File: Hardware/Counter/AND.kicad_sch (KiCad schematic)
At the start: 6 parts, among them Q105 FDN360P, Q106 FDN335N, Q107 FDN335N, Q108 FDN335N, U60 FDN360P, U61 FDN360P

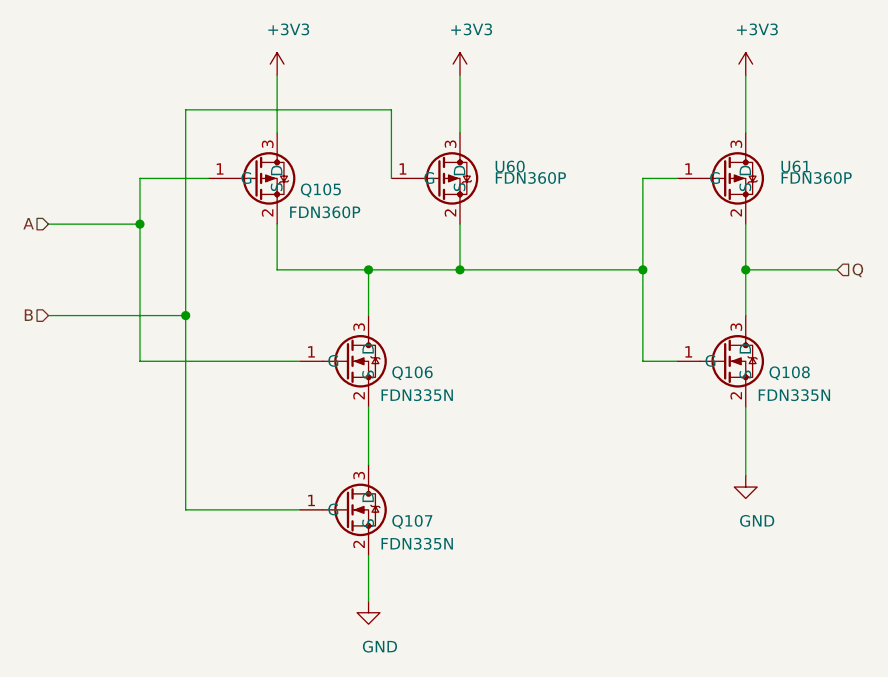
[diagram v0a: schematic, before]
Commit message: working on connectin bits together
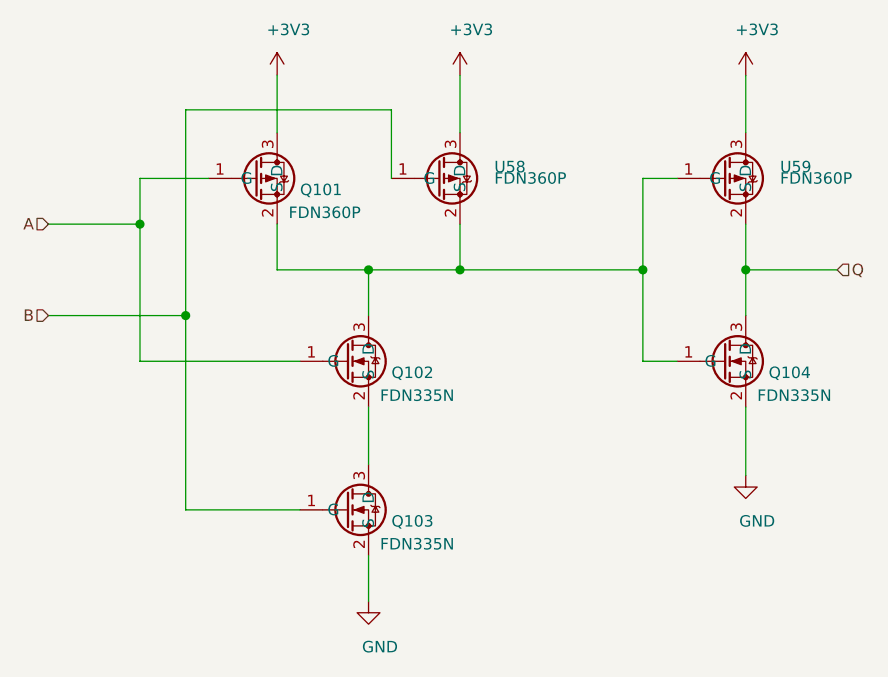
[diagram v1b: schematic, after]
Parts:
- renumbered Q105 to Q101, Q106 to Q102, Q107 to Q103, Q108 to Q104, U60 to U58, U61 to U59
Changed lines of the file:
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@@
   (symbol (lib_id "power:+3V3") (at 124.46 64.77 0)
     (in_bom yes) (on_board yes)
-    (property "Reference" "#PWR0233" (id 0) (at 124.46 68.58 0)
+    (property "Reference" "#PWR0228" (id 0) (at 124.46 68.58 0)
       (effects (font (size 1.27 1.27)) hide)
     )
@@
   (symbol (lib_id "power:+3V3") (at 144.78 64.77 0)
     (in_bom yes) (on_board yes)
-    (property "Reference" "#PWR0234" (id 0) (at 144.78 68.58 0)
+    (property "Reference" "#PWR0229" (id 0) (at 144.78 68.58 0)
       (effects (font (size 1.27 1.27)) hide)
     )
@@
   (symbol (lib_id "power:+3V3") (at 176.53 64.77 0)
     (in_bom yes) (on_board yes)
-    (property "Reference" "#PWR0235" (id 0) (at 176.53 68.58 0)
+    (property "Reference" "#PWR0230" (id 0) (at 176.53 68.58 0)
       (effects (font (size 1.27 1.27)) hide)
     )
@@
   (symbol (lib_id "power:GND") (at 134.62 123.19 0)
     (in_bom yes) (on_board yes)
-    (property "Reference" "#PWR0231" (id 0) (at 134.62 129.54 0)
+    (property "Reference" "#PWR0226" (id 0) (at 134.62 129.54 0)
       (effects (font (size 1.27 1.27)) hide)
     )
@@
   (symbol (lib_id "power:GND") (at 176.53 109.22 0)
     (in_bom yes) (on_board yes)
-    (property "Reference" "#PWR0232" (id 0) (at 176.53 115.57 0)
+    (property "Reference" "#PWR0227" (id 0) (at 176.53 115.57 0)
       (effects (font (size 1.27 1.27)) hide)
     )
@@
   (symbol (lib_name "Custom_Transistors:FDN360P_1") (lib_id "Custom_Transistors:FDN360P") (at 124.46 76.2 0)
     (in_bom yes) (on_board yes)
-    (property "Reference" "Q105" (id 0) (at 127 77.47 0)
+    (property "Reference" "Q101" (id 0) (at 127 77.47 0)
       (effects (font (size 1.27 1.27)) (justify left))
     )
@@
   (symbol (lib_id "Custom_Transistors:FDN335N") (at 134.62 96.52 0)
     (in_bom yes) (on_board yes)
-    (property "Reference" "Q106" (id 0) (at 137.16 97.79 0)
+    (property "Reference" "Q102" (id 0) (at 137.16 97.79 0)
       (effects (font (size 1.27 1.27)) (justify left))
     )
@@
   (symbol (lib_id "Custom_Transistors:FDN335N") (at 134.62 113.03 0)
     (in_bom yes) (on_board yes)
-    (property "Reference" "Q107" (id 0) (at 137.16 114.3 0)
+    (property "Reference" "Q103" (id 0) (at 137.16 114.3 0)
       (effects (font (size 1.27 1.27)) (justify left))
     )
@@
   (symbol (lib_name "Custom_Transistors:FDN360P_2") (lib_id "Custom_Transistors:FDN360P") (at 144.78 76.2 0)
     (in_bom yes) (on_board yes)
-    (property "Reference" "U60" (id 0) (at 148.59 74.93 0)
+    (property "Reference" "U58" (id 0) (at 148.59 74.93 0)
       (effects (font (size 1.27 1.27)) (justify left))
     )
@@
   (symbol (lib_id "Custom_Transistors:FDN360P") (at 176.53 76.2 0)
     (in_bom yes) (on_board yes)
-    (property "Reference" "U61" (id 0) (at 180.34 74.93 0)
+    (property "Reference" "U59" (id 0) (at 180.34 74.93 0)
       (effects (font (size 1.27 1.27)) (justify left))
     )
@@
   (symbol (lib_id "Custom_Transistors:FDN335N") (at 176.53 96.52 0)
     (in_bom yes) (on_board yes)
-    (property "Reference" "Q108" (id 0) (at 179.07 97.79 0)
+    (property "Reference" "Q104" (id 0) (at 179.07 97.79 0)
       (effects (font (size 1.27 1.27)) (justify left))
     )

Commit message: kicad updates
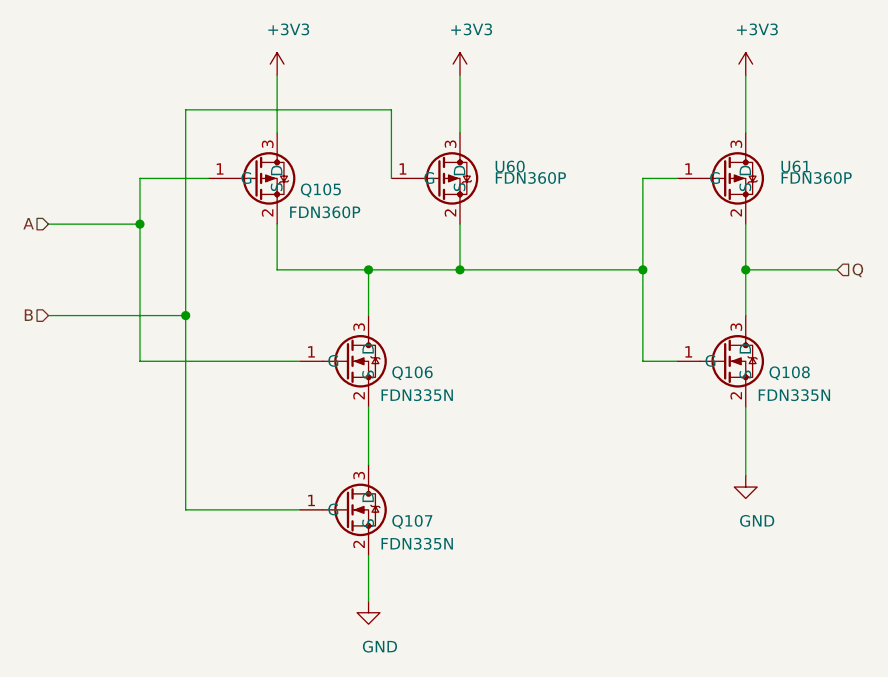
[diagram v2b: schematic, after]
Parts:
- renumbered Q101 to Q105, Q102 to Q106, Q103 to Q107, Q104 to Q108, U58 to U60, U59 to U61
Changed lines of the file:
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@@
   (symbol (lib_id "power:+3V3") (at 124.46 64.77 0)
     (in_bom yes) (on_board yes)
-    (property "Reference" "#PWR0228" (id 0) (at 124.46 68.58 0)
+    (property "Reference" "#PWR0233" (id 0) (at 124.46 68.58 0)
       (effects (font (size 1.27 1.27)) hide)
     )
@@
   (symbol (lib_id "power:+3V3") (at 144.78 64.77 0)
     (in_bom yes) (on_board yes)
-    (property "Reference" "#PWR0229" (id 0) (at 144.78 68.58 0)
+    (property "Reference" "#PWR0234" (id 0) (at 144.78 68.58 0)
       (effects (font (size 1.27 1.27)) hide)
     )
@@
   (symbol (lib_id "power:+3V3") (at 176.53 64.77 0)
     (in_bom yes) (on_board yes)
-    (property "Reference" "#PWR0230" (id 0) (at 176.53 68.58 0)
+    (property "Reference" "#PWR0235" (id 0) (at 176.53 68.58 0)
       (effects (font (size 1.27 1.27)) hide)
     )
@@
   (symbol (lib_id "power:GND") (at 134.62 123.19 0)
     (in_bom yes) (on_board yes)
-    (property "Reference" "#PWR0226" (id 0) (at 134.62 129.54 0)
+    (property "Reference" "#PWR0231" (id 0) (at 134.62 129.54 0)
       (effects (font (size 1.27 1.27)) hide)
     )
@@
   (symbol (lib_id "power:GND") (at 176.53 109.22 0)
     (in_bom yes) (on_board yes)
-    (property "Reference" "#PWR0227" (id 0) (at 176.53 115.57 0)
+    (property "Reference" "#PWR0232" (id 0) (at 176.53 115.57 0)
       (effects (font (size 1.27 1.27)) hide)
     )
@@
   (symbol (lib_name "Custom_Transistors:FDN360P_1") (lib_id "Custom_Transistors:FDN360P") (at 124.46 76.2 0)
     (in_bom yes) (on_board yes)
-    (property "Reference" "Q101" (id 0) (at 127 77.47 0)
+    (property "Reference" "Q105" (id 0) (at 127 77.47 0)
       (effects (font (size 1.27 1.27)) (justify left))
     )
@@
   (symbol (lib_id "Custom_Transistors:FDN335N") (at 134.62 96.52 0)
     (in_bom yes) (on_board yes)
-    (property "Reference" "Q102" (id 0) (at 137.16 97.79 0)
+    (property "Reference" "Q106" (id 0) (at 137.16 97.79 0)
       (effects (font (size 1.27 1.27)) (justify left))
     )
@@
   (symbol (lib_id "Custom_Transistors:FDN335N") (at 134.62 113.03 0)
     (in_bom yes) (on_board yes)
-    (property "Reference" "Q103" (id 0) (at 137.16 114.3 0)
+    (property "Reference" "Q107" (id 0) (at 137.16 114.3 0)
       (effects (font (size 1.27 1.27)) (justify left))
     )
@@
   (symbol (lib_name "Custom_Transistors:FDN360P_2") (lib_id "Custom_Transistors:FDN360P") (at 144.78 76.2 0)
     (in_bom yes) (on_board yes)
-    (property "Reference" "U58" (id 0) (at 148.59 74.93 0)
+    (property "Reference" "U60" (id 0) (at 148.59 74.93 0)
       (effects (font (size 1.27 1.27)) (justify left))
     )
@@
   (symbol (lib_id "Custom_Transistors:FDN360P") (at 176.53 76.2 0)
     (in_bom yes) (on_board yes)
-    (property "Reference" "U59" (id 0) (at 180.34 74.93 0)
+    (property "Reference" "U61" (id 0) (at 180.34 74.93 0)
       (effects (font (size 1.27 1.27)) (justify left))
     )
@@
   (symbol (lib_id "Custom_Transistors:FDN335N") (at 176.53 96.52 0)
     (in_bom yes) (on_board yes)
-    (property "Reference" "Q104" (id 0) (at 179.07 97.79 0)
+    (property "Reference" "Q108" (id 0) (at 179.07 97.79 0)
       (effects (font (size 1.27 1.27)) (justify left))
     )
